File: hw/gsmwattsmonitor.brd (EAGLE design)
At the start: 55 x 80 mm, 9 parts

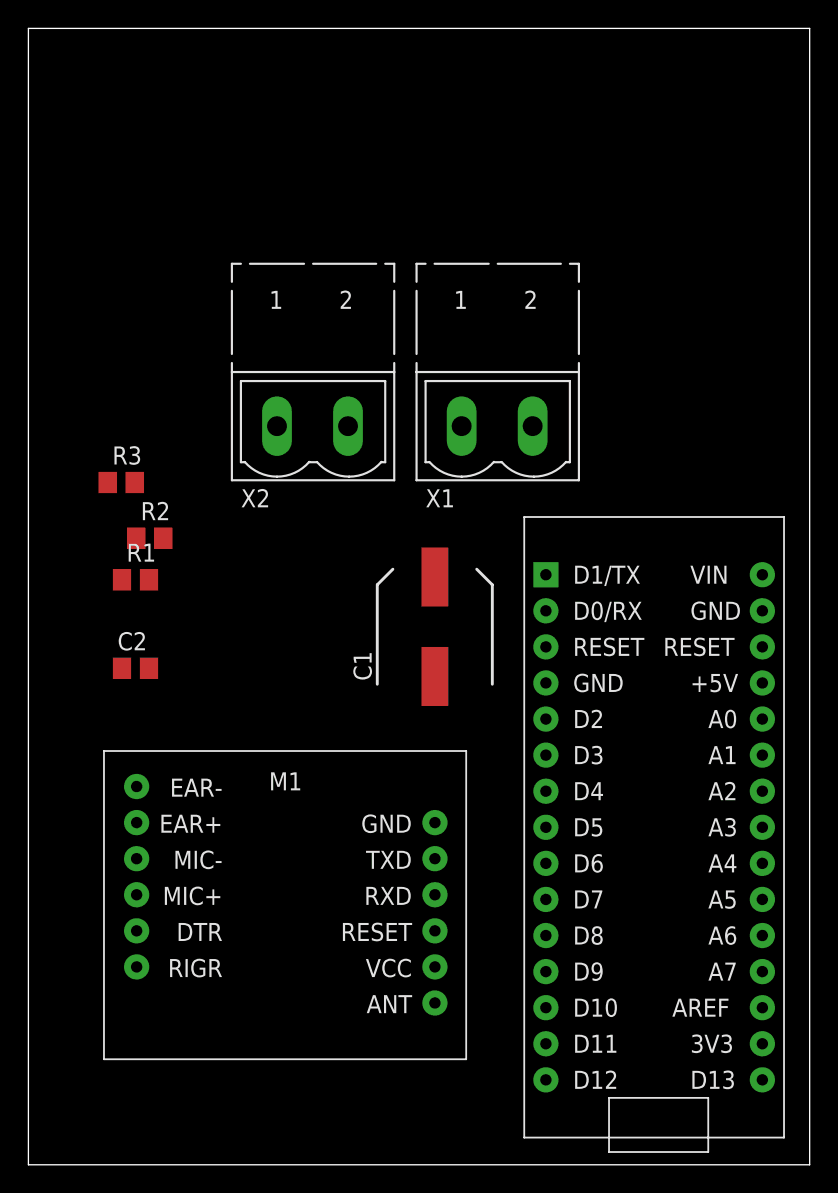
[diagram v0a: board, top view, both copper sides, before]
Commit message: updated hardware
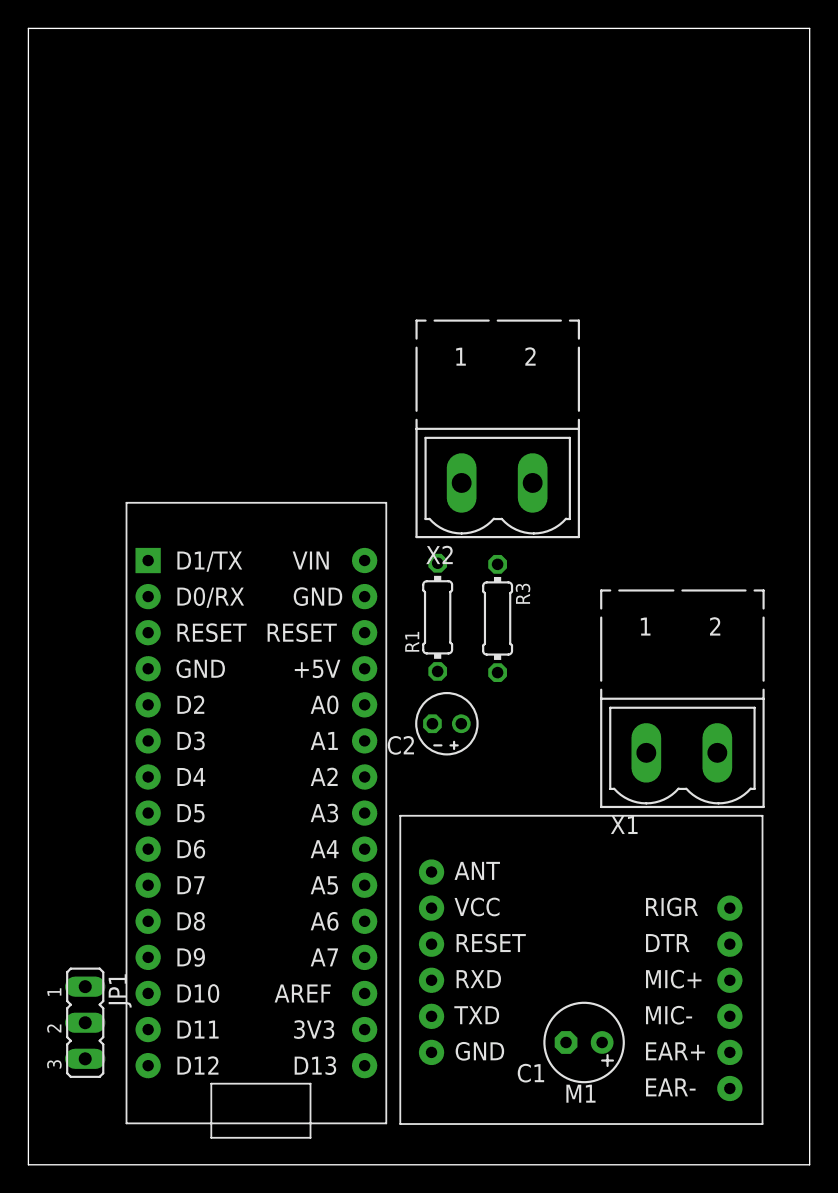
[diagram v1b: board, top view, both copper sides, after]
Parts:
- removed R2: 33R, rcl:R0805
- added JP1: (no value), jumper:JP2
- C1: device rcl:SANYO-OSCON_SMD_E7 -> rcl:E2,5-6
- C2: device rcl:C0805 -> rcl:E2-4
- R1, R3: device rcl:R0805 -> rcl:0204/7
- moved C1 31.1 mm to (39.1, 8.61), turned to 180 degrees
- moved R3 28.2 mm to (33.0, 38.5), turned to 270 degrees
- moved U$1 28.0 mm to (16.1, 24.8)
- moved X1 26.4 mm to (46.0, 29.0)
- moved C2 22.3 mm to (29.5, 31.1), turned to 180 degrees
- moved M1 21.6 mm to (38.9, 13.1), turned to 0 degrees
- moved R1 21.4 mm to (28.8, 38.5), turned to 90 degrees
- moved X2 13.6 mm to (33.0, 48.0)
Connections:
- new net N$2: JP1.3, U$1.D12
- net +3V3: now also R3.2; no longer R1.2
- net CURRENT_PIN: now also U$1.A1, X2.2; no longer R2.2, U$1.A0, X2.1
- net GND: now also C2.-, JP1.1, R1.1; no longer C2.1, R3.1
- net GSM_RST: now also U$1.D7; no longer U$1.D4
- net GSM_RXD: now also U$1.D8; no longer U$1.D2
- net GSM_TXD: now also U$1.D9; no longer U$1.D3
- net N$1: now also C2.+, R1.2, R3.1, X2.1; no longer C2.2, R1.1, R2.1, R3.2, X2.2
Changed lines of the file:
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@@
 </autorouter>
 <elements>
-<element name="U$1" library="rocketfarm" package="PDIP-32" value="" x="44.05" y="23.76" smashed="yes"/>
-<element name="C1" library="rcl" package="SANYO-OSCON_SMD_E7" value="470u" x="28.61" y="37.88" rot="R90"/>
-<element name="M1" library="library" package="SIM800L" value="" x="18.12" y="18.93" smashed="yes" rot="R180">
-<attribute name="NAME" x="19.28" y="27.63" size="1.27" layer="25" rot="R180"/>
-<attribute name="VALUE" x="28.28" y="34.17" size="1.27" layer="27" rot="R180"/>
+<element name="U$1" library="rocketfarm" package="PDIP-32" value="" x="16.05" y="24.76" smashed="yes"/>
+<element name="C1" library="rcl" package="E2,5-6" value="470u" x="39.12" y="8.61" rot="R180"/>
+<element name="M1" library="library" package="SIM800L" value="" x="38.88" y="13.07" smashed="yes">
+<attribute name="NAME" x="37.72" y="4.37" size="1.27" layer="25"/>
+<attribute name="VALUE" x="28.72" y="-2.17" size="1.27" layer="27"/>
 </element>
-<element name="R1" library="rcl" package="R0805" value="10k" x="7.54" y="41.19"/>
-<element name="R2" library="rcl" package="R0805" value="33R" x="8.54" y="44.11"/>
-<element name="R3" library="rcl" package="R0805" value="10k" x="6.54" y="48.03"/>
-<element name="C2" library="rcl" package="C0805" value="10u" x="7.54" y="34.95"/>
-<element name="X1" library="con-phoenix-500" package="MSTBV2" value="" x="33" y="52">
-<attribute name="OC_NEWARK" value="unknown" x="33" y="52" size="1.778" layer="27" display="off"/>
-<attribute name="MPN" value="" x="33" y="52" size="1.778" layer="27" display="off"/>
-<attribute name="MF" value="" x="33" y="52" size="1.778" layer="27" display="off"/>
-<attribute name="OC_FARNELL" value="unknown" x="33" y="52" size="1.778" layer="27" display="off"/>
+<element name="R1" library="rcl" package="0204/7" value="10k" x="28.81" y="38.54" rot="R90"/>
+<element name="R3" library="rcl" package="0204/7" value="10k" x="33.03" y="38.46" rot="R270"/>
+<element name="C2" library="rcl" package="E2-4" value="10u" x="29.46" y="31.05" rot="R180"/>
+<element name="X1" library="con-phoenix-500" package="MSTBV2" value="" x="46" y="29">
+<attribute name="OC_NEWARK" value="unknown" x="46" y="29" size="1.778" layer="27" display="off"/>
+<attribute name="MPN" value="" x="46" y="29" size="1.778" layer="27" display="off"/>
+<attribute name="MF" value="" x="46" y="29" size="1.778" layer="27" display="off"/>
+<attribute name="OC_FARNELL" value="unknown" x="46" y="29" size="1.778" layer="27" display="off"/>
 </element>
-<element name="X2" library="con-phoenix-500" package="MSTBV2" value="" x="20" y="52">
-<attribute name="OC_NEWARK" value="unknown" x="20" y="52" size="1.778" layer="27" display="off"/>
-<attribute name="MPN" value="" x="20" y="52" size="1.778" layer="27" display="off"/>
-<attribute name="MF" value="" x="20" y="52" size="1.778" layer="27" display="off"/>
-<attribute name="OC_FARNELL" value="unknown" x="20" y="52" size="1.778" layer="27" display="off"/>
+<element name="X2" library="con-phoenix-500" package="MSTBV2" value="" x="33" y="48">
+<attribute name="OC_NEWARK" value="unknown" x="33" y="48" size="1.778" layer="27" display="off"/>
+<attribute name="MPN" value="" x="33" y="48" size="1.778" layer="27" display="off"/>
+<attribute name="MF" value="" x="33" y="48" size="1.778" layer="27" display="off"/>
+<attribute name="OC_FARNELL" value="unknown" x="33" y="48" size="1.778" layer="27" display="off"/>
 </element>
+<element name="JP1" library="jumper" package="JP2" value="" x="4" y="10" rot="R270"/>
 </elements>
 <signals>
@@
 <contactref element="M1" pad="VCC"/>
 <contactref element="X1" pad="2"/>
-<wire x1="28.61" y1="41.38" x2="35.5" y2="52" width="0" layer="19" extent="1-1"/>
-<wire x1="28.62" y1="13.93" x2="28.61" y2="41.38" width="0" layer="19" extent="1-1"/>
-<wire x1="51.67" y1="33.92" x2="28.62" y2="13.93" width="0" layer="19" extent="1-1"/>
+<wire x1="40.39" y1="8.61" x2="48.5" y2="29" width="0" layer="19" extent="1-1"/>
+<wire x1="28.38" y1="18.07" x2="40.39" y2="8.61" width="0" layer="19" extent="1-1"/>
+<wire x1="23.67" y1="34.92" x2="28.38" y2="18.07" width="0" layer="19" extent="1-1"/>
 </signal>
 <signal name="GND">
@@
 <contactref element="U$1" pad="GND1"/>
 <contactref element="C1" pad="-"/>
-<contactref element="R3" pad="1"/>
-<contactref element="C2" pad="1"/>
 <contactref element="M1" pad="GND"/>
 <contactref element="X1" pad="1"/>
-<wire x1="28.61" y1="34.38" x2="30.5" y2="52" width="0" layer="19" extent="1-1"/>
-<wire x1="36.43" y1="33.92" x2="28.61" y2="34.38" width="0" layer="19" extent="1-1"/>
-<wire x1="51.67" y1="39" x2="36.43" y2="33.92" width="0" layer="19" extent="1-1"/>
-<wire x1="28.62" y1="24.09" x2="36.43" y2="33.92" width="0" layer="19" extent="1-1"/>
-<wire x1="6.59" y1="34.95" x2="28.61" y2="34.38" width="0" layer="19" extent="1-1"/>
-<wire x1="5.59" y1="48.03" x2="6.59" y2="34.95" width="0" layer="19" extent="1-1"/>
-</signal>
-<signal name="N$1">
 <contactref element="R1" pad="1"/>
-<contactref element="R3" pad="2"/>
-<contactref element="C2" pad="2"/>
-<contactref element="R2" pad="1"/>
-<contactref element="X2" pad="2"/>
-<wire x1="7.49" y1="48.03" x2="6.59" y2="41.19" width="0" layer="19" extent="1-1"/>
-<wire x1="8.49" y1="34.95" x2="7.49" y2="48.03" width="0" layer="19" extent="1-1"/>
-<wire x1="7.59" y1="44.11" x2="8.49" y2="34.95" width="0" layer="19" extent="1-1"/>
-<wire x1="22.5" y1="52" x2="7.49" y2="48.03" width="0" layer="19" extent="1-1"/>
+<contactref element="C2" pad="-"/>
+<contactref element="JP1" pad="1"/>
+<wire x1="28.444" y1="31.05" x2="43.5" y2="29" width="0" layer="19" extent="1-1"/>
+<wire x1="28.81" y1="34.73" x2="28.444" y2="31.05" width="0" layer="19" extent="1-1"/>
+<wire x1="23.67" y1="40" x2="28.81" y2="34.73" width="0" layer="19" extent="1-1"/>
+<wire x1="8.43" y1="34.92" x2="23.67" y2="40" width="0" layer="19" extent="1-1"/>
+<wire x1="37.85" y1="8.61" x2="43.5" y2="29" width="0" layer="19" extent="1-1"/>
+<wire x1="28.38" y1="7.91" x2="37.85" y2="8.61" width="0" layer="19" extent="1-1"/>
+<wire x1="4" y1="12.54" x2="8.43" y2="34.92" width="0" layer="19" extent="1-1"/>
 </signal>
 <signal name="+3V3">
 <contactref element="U$1" pad="3V3"/>
-<contactref element="R1" pad="2"/>
-<wire x1="51.67" y1="8.52" x2="8.49" y2="41.19" width="0" layer="19" extent="1-1"/>
+<contactref element="R3" pad="2"/>
+<wire x1="23.67" y1="9.52" x2="33.03" y2="34.65" width="0" layer="19" extent="1-1"/>
 </signal>
 <signal name="CURRENT_PIN">
-<contactref element="R2" pad="2"/>
-<contactref element="U$1" pad="A0"/>
-<contactref element="X2" pad="1"/>
-<wire x1="17.5" y1="52" x2="9.49" y2="44.11" width="0" layer="19" extent="1-1"/>
-<wire x1="51.67" y1="31.38" x2="17.5" y2="52" width="0" layer="19" extent="1-1"/>
+<contactref element="X2" pad="2"/>
+<contactref element="U$1" pad="A1"/>
+<wire x1="23.67" y1="29.84" x2="35.5" y2="48" width="0" layer="19" extent="1-1"/>
 </signal>
 <signal name="GSM_RST">
 <contactref element="M1" pad="RESET"/>
-<contactref element="U$1" pad="D4"/>
-<wire x1="28.62" y1="16.47" x2="36.43" y2="26.3" width="0" layer="19" extent="1-1"/>
+<contactref element="U$1" pad="D7"/>
+<wire x1="8.43" y1="19.68" x2="28.38" y2="15.53" width="0" layer="19" extent="1-1"/>
 </signal>
 <signal name="GSM_RXD">
 <contactref element="M1" pad="RXD"/>
-<contactref element="U$1" pad="D2"/>
-<wire x1="28.62" y1="19.01" x2="36.43" y2="31.38" width="0" layer="19" extent="1-1"/>
+<contactref element="U$1" pad="D8"/>
+<wire x1="8.43" y1="17.14" x2="28.38" y2="12.99" width="0" layer="19" extent="1-1"/>
 </signal>
 <signal name="GSM_TXD">
 <contactref element="M1" pad="TXD"/>
-<contactref element="U$1" pad="D3"/>
-<wire x1="28.62" y1="21.55" x2="36.43" y2="28.84" width="0" layer="19" extent="1-1"/>
+<contactref element="U$1" pad="D9"/>
+<wire x1="8.43" y1="14.6" x2="28.38" y2="10.45" width="0" layer="19" extent="1-1"/>
+</signal>
+<signal name="N$1">
+<contactref element="X2" pad="1"/>
+<contactref element="C2" pad="+"/>
+<contactref element="R3" pad="1"/>
+<contactref element="R1" pad="2"/>
+<wire x1="28.81" y1="42.35" x2="30.5" y2="48" width="0" layer="19" extent="1-1"/>
+<wire x1="33.03" y1="42.27" x2="28.81" y2="42.35" width="0" layer="19" extent="1-1"/>
+<wire x1="30.476" y1="31.05" x2="28.81" y2="42.35" width="0" layer="19" extent="1-1"/>
+</signal>
+<signal name="N$2">
+<contactref element="U$1" pad="D12"/>
+<contactref element="JP1" pad="3"/>
+<wire x1="4" y1="7.46" x2="8.43" y2="6.98" width="0" layer="19" extent="1-1"/>
 </signal>
 </signals>
